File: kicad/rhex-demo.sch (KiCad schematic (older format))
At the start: 24 parts

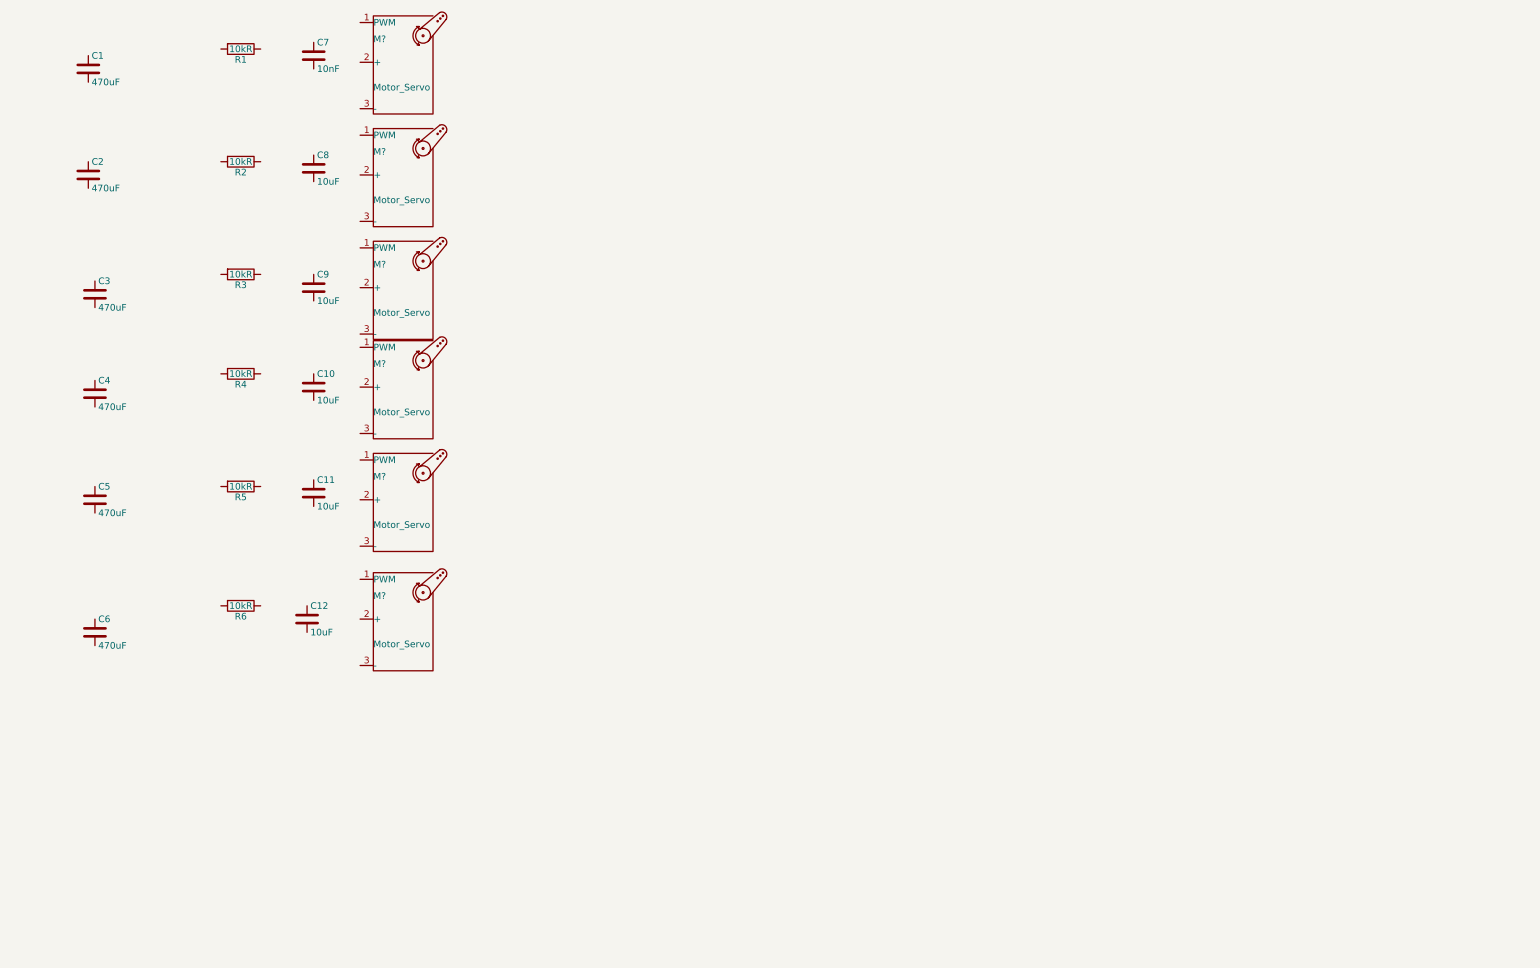
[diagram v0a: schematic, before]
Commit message: main thread for testing
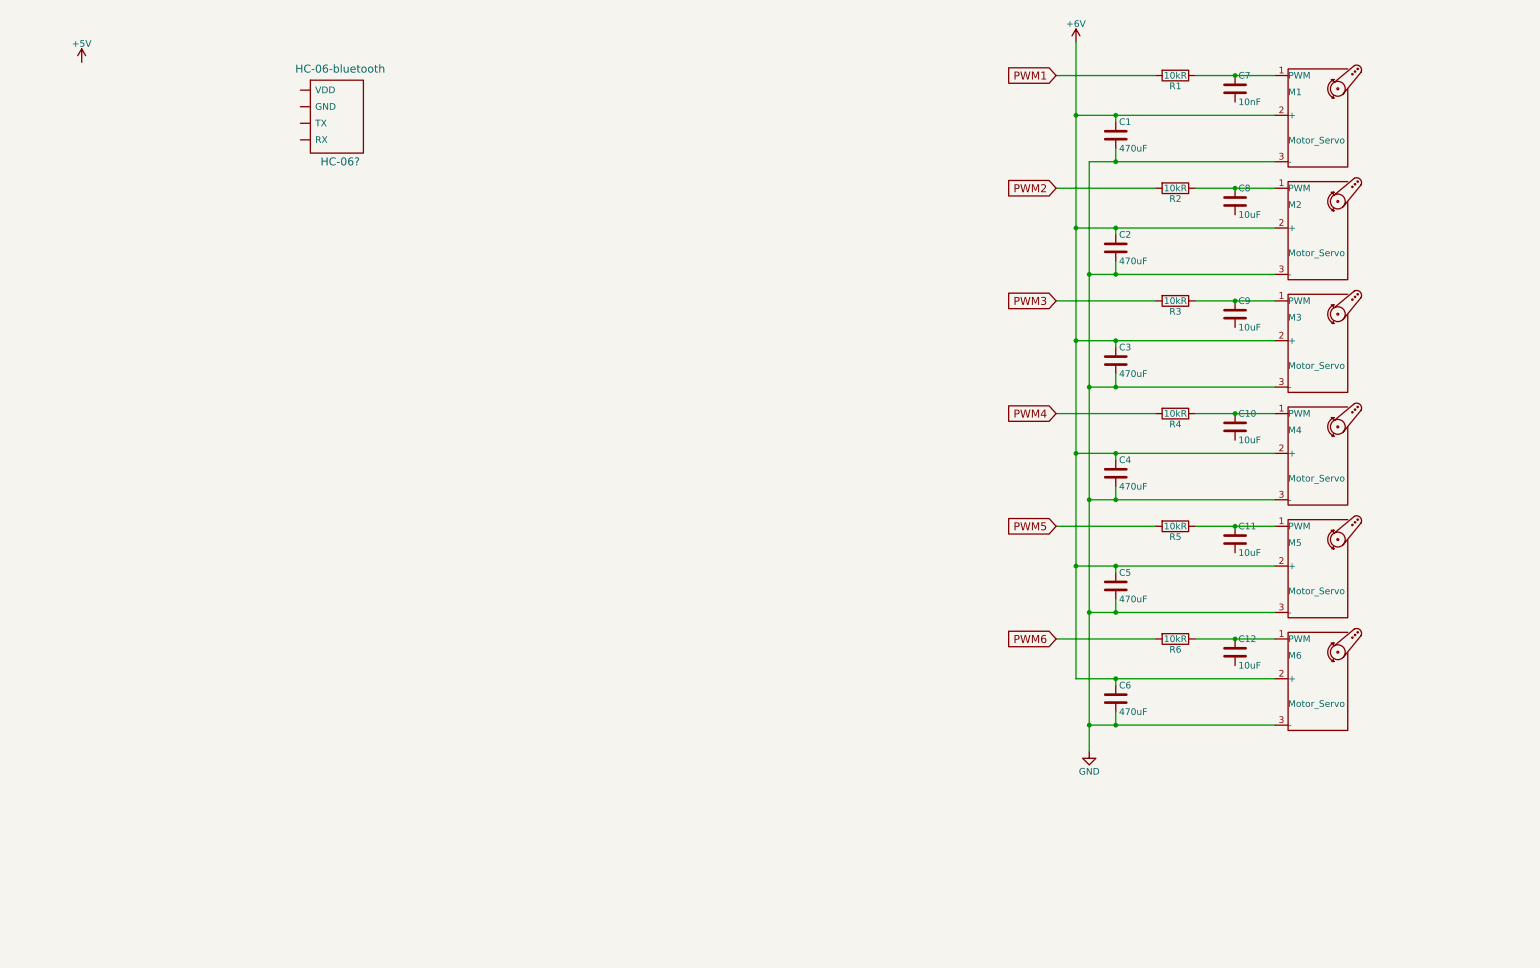
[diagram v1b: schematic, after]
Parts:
- added HC-06?: HC-06-bluetooth, symbol HC-06-bluetooth
- gave numbers to parts that had none: 6
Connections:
- net at M1.1 (PWM): now also C7.1, R1.1
- net +6V: now reaches M1.2 (+)
- net +6V: now also C1.1, C2.1, C3.1, C4.1, C5.1, C6.1, M2.2 (+), M3.2 (+), M4.2 (+), M5.2 (+), M6.2 (+)
- net GND: now reaches M1.3 (-)
- net GND: now also C1.2, C2.2, C3.2, C4.2, C5.2, C6.2, M2.3 (-), M3.3 (-), M4.3 (-), M5.3 (-), M6.3 (-)
- net at M2.1 (PWM): now also C8.1, R2.1
- net at M3.1 (PWM): now also C9.1, R3.1
- net at M4.1 (PWM): now also C10.1, R4.1
- net at M5.1 (PWM): now also C11.1, R5.1
- net at M6.1 (PWM): now also C12.1, R6.1
- net PWM1: now reaches R1.2
- net PWM2: now reaches R2.2
- net PWM3: now reaches R3.2
- net PWM4: now reaches R4.2
- net PWM5: now reaches R5.2
- net PWM6: now reaches R6.2
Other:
- moved on the sheet: C1, C10, C11, C12, C2, C3, C4, C5, C6, C7, C8, C9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

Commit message: layout half done
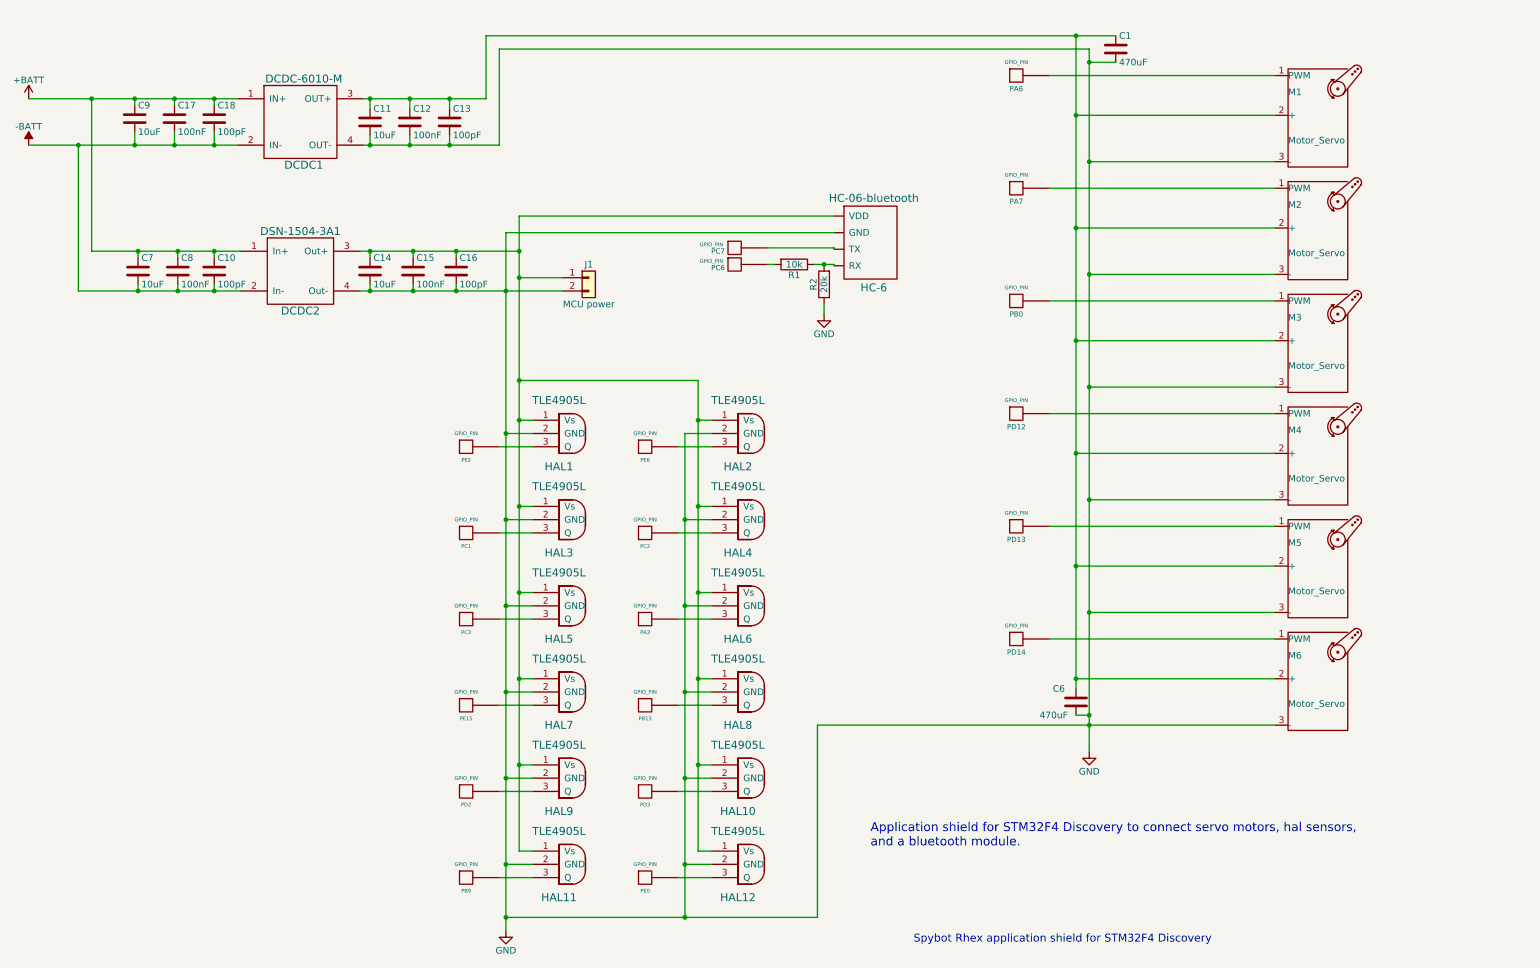
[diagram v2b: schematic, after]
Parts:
- removed C2, C3, C4, C5: 470uF, symbol C
- removed HC-06?: HC-06-bluetooth, symbol HC-06-bluetooth
- removed R3, R4, R5, R6: 10kR, symbol R
- added C13, C16, C18: 100pF, Capacitors_THT:C_Axial_L3.8mm_D2.6mm_P7.50mm_Horizontal, symbol C
- added C14: 10uF, Capacitors_THT:C_Axial_L3.8mm_D2.6mm_P7.50mm_Horizontal, symbol C
- added C15, C17: 100nF, Capacitors_THT:C_Axial_L3.8mm_D2.6mm_P7.50mm_Horizontal, symbol C
- added DCDC1: DCDC-6010-M, rhex:DCDC-6010-M, symbol DCDC-6010-M
- added DSN-1504-3A1: DCDC2, rhex2:DSN-1504-2A1, symbol DSN-1504-3A
- added HAL1, HAL10, HAL11, HAL12, HAL2, HAL3, HAL4, HAL5, HAL6, HAL7, HAL8, HAL9: TLE4905L, Pin_Headers:Pin_Header_Straight_1x03_Pitch2.54mm, symbol TLE4905L
- added HC-6: HC-06-bluetooth, Pin_Headers:Pin_Header_Straight_1x06_Pitch2.54mm, symbol HC-06-bluetooth
- added J1: MCU power, Pin_Headers:Pin_Header_Straight_1x02_Pitch2.54mm, symbol Conn_01x02
- added PA3, PA6, PA7, PB0, PB13, PB9, PC1, PC2, PC3, PC6, PC7, PD12, PD13, PD14, PD2, PD3, PE0, PE15, PE2, PE6: GPIO_PIN, Pin_Headers:Pin_Header_Straight_1x01_Pitch2.54mm, symbol GPIO_PIN
- C1, C11, C6, C9: footprint (none) -> Capacitors_THT:C_Axial_L3.8mm_D2.6mm_P7.50mm_Horizontal
- C10: value 10uF -> 100pF; footprint (none) -> Capacitors_THT:C_Axial_L3.8mm_D2.6mm_P7.50mm_Horizontal
- C12, C8: value 10uF -> 100nF; footprint (none) -> Capacitors_THT:C_Axial_L3.8mm_D2.6mm_P7.50mm_Horizontal
- C7: value 10nF -> 10uF; footprint (none) -> Capacitors_THT:C_Axial_L3.8mm_D2.6mm_P7.50mm_Horizontal
- M1, M2, M3, M4, M5, M6: footprint (none) -> Pin_Headers:Pin_Header_Straight_1x03_Pitch2.54mm
- R1: value 10kR -> 10k; footprint (none) -> Resistors_THT:R_Axial_DIN0204_L3.6mm_D1.6mm_P5.08mm_Horizontal
- R2: value 10kR -> 20k; footprint (none) -> Resistors_THT:R_Axial_DIN0204_L3.6mm_D1.6mm_P5.08mm_Horizontal
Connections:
- net +6V is gone; now on an unnamed net: C1.1, C6.1, M1.2 (+), M2.2 (+), M3.2 (+), M4.2 (+), M5.2 (+), M6.2 (+)
- net GND: now also C11.2, C12.2, R2.1, C13.2, C14.2, C15.2, C16.2, DCDC1.4 (OUT-), DSN-1504-3A1.4 (Out-), HAL1.2 (GND), HAL10.2 (GND), HAL11.2 (GND), HAL12.2 (GND), HAL2.2 (GND), HAL3.2 (GND), HAL4.2 (GND), HAL5.2 (GND), HAL6.2 (GND), HAL7.2 (GND), HAL8.2 (GND), HAL9.2 (GND), HC-6.~ (VDD), J1.2 (Pin_2)
- net at M3.1 (PWM): now also PB0.~; no longer C9.1
- net at M4.1 (PWM): now also PD12.~; no longer C10.1
- net at C11.1: now also C12.1, C13.1, DCDC1.3 (OUT+); no longer M5.1 (PWM)
- net at M6.1 (PWM): now also PD14.~; no longer C12.1
- net -BATT: now reaches C8.2
- net -BATT: now also C10.2, C7.2, C9.2, C17.2, C18.2, DCDC1.2 (IN-), DSN-1504-3A1.2 (In-)
- net PWM1: no longer names the net of R1.2
- net PWM1: now also PC6.~
- net PWM2: no longer names the net of R2.2
- net PWM2: now also R1.1, HC-6.~ (VDD)
- new net: M1.1 (PWM), PA6.~
- new net: M2.1 (PWM), PA7.~
- new net: M5.1 (PWM), PD13.~
- new net: C14.1, C15.1, C16.1, DSN-1504-3A1.3 (Out+), HAL1.1 (Vs), HAL10.1 (Vs), HAL11.1 (Vs), HAL12.1 (Vs), HAL2.1 (Vs), HAL3.1 (Vs), HAL4.1 (Vs), HAL5.1 (Vs), HAL6.1 (Vs), HAL7.1 (Vs), HAL8.1 (Vs), HAL9.1 (Vs), HC-6.~ (VDD), J1.1 (Pin_1)
- new net: HAL1.3 (Q), PE2.~
- new net: HAL3.3 (Q), PC1.~
- new net: HAL5.3 (Q), PC3.~
- new net: HAL7.3 (Q), PE15.~
- new net: HAL9.3 (Q), PD2.~
- new net: HAL11.3 (Q), PB9.~
- new net: HAL2.3 (Q), PE6.~
- new net: HAL4.3 (Q), PC2.~
- new net: HAL6.3 (Q), PA3.~
- new net: HAL8.3 (Q), PB13.~
- new net: HAL10.3 (Q), PD3.~
- new net: HAL12.3 (Q), PE0.~
- new net: HC-6.~ (VDD), PC7.~
- new net +BATT: C10.1, C17.1, C18.1, C7.1, C8.1, C9.1, DCDC1.1 (IN+), DSN-1504-3A1.1 (In+)
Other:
- note added: "Application shield for STM32F4 Discovery to connect servo motors, hal sensors,\nand a bluetooth module."
- note added: "Spybot Rhex application shield for STM32F4 Discovery"
- moved on the sheet: C1, C6
